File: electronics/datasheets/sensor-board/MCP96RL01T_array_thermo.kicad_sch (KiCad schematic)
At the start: 75 parts, among them J23 Therm_1, J24 Therm_4, J25 Therm_7, J26 Therm_2, J27 Therm_5, J28 Therm_3, J29 Therm_6, U10 MCP96RL01T, U4 MCP96RL01T, U5 MCP96RL01T, U6 MCP96RL01T, U7 MCP96RL01T, U8 MCP96RL01T, U9 MCP96RL01T

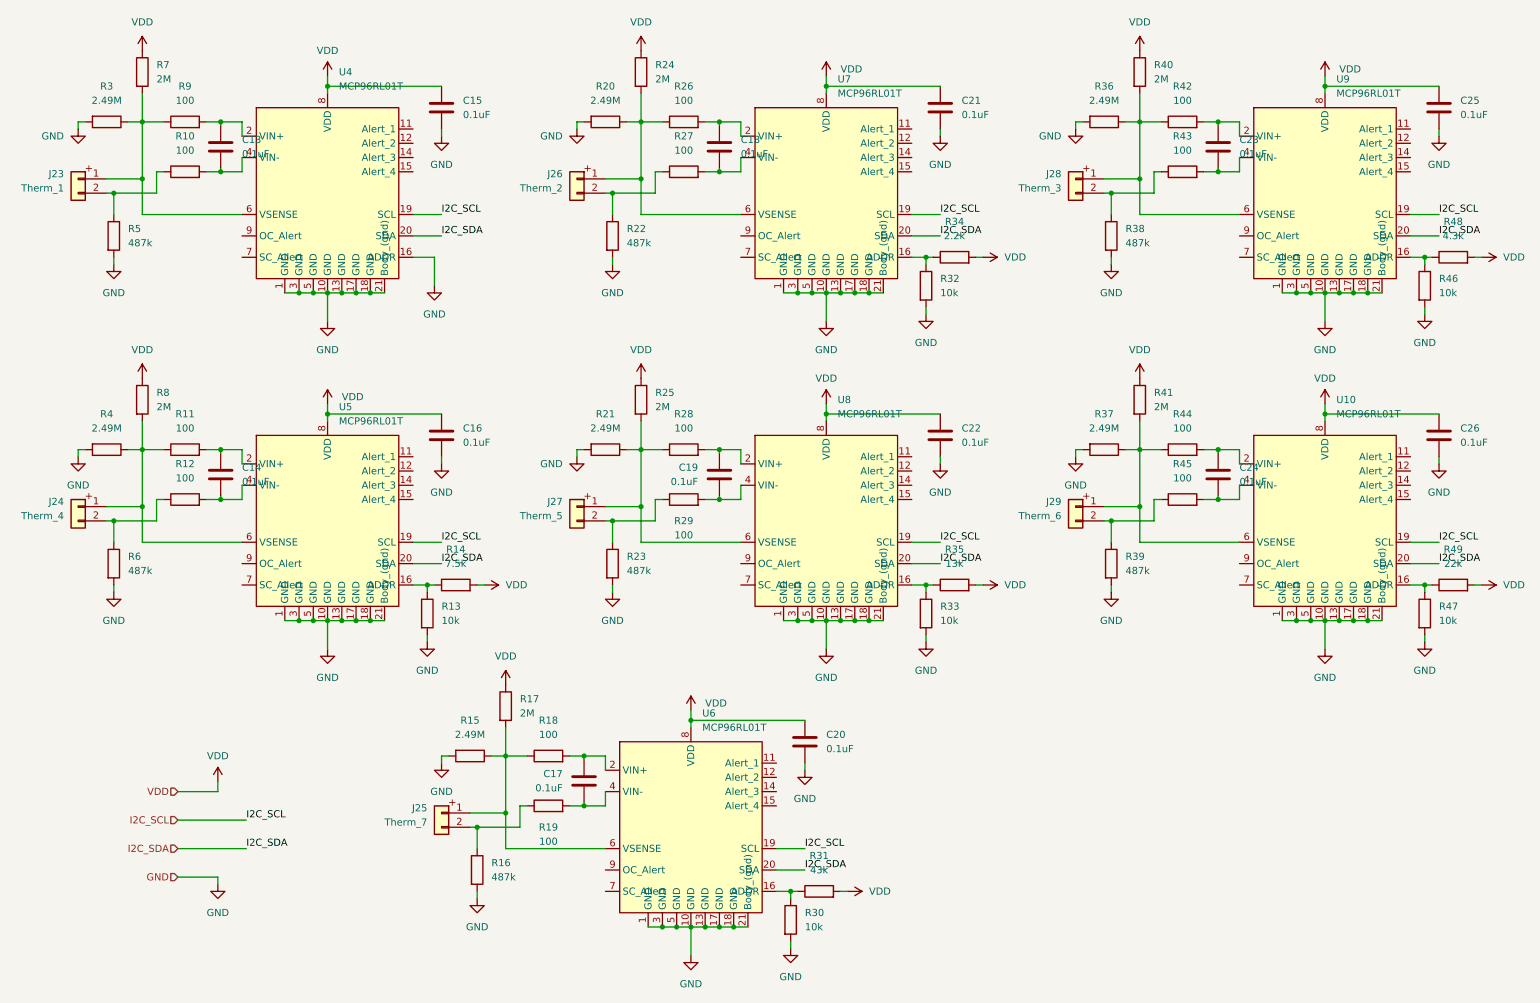
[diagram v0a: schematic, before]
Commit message: Work on sensor-board
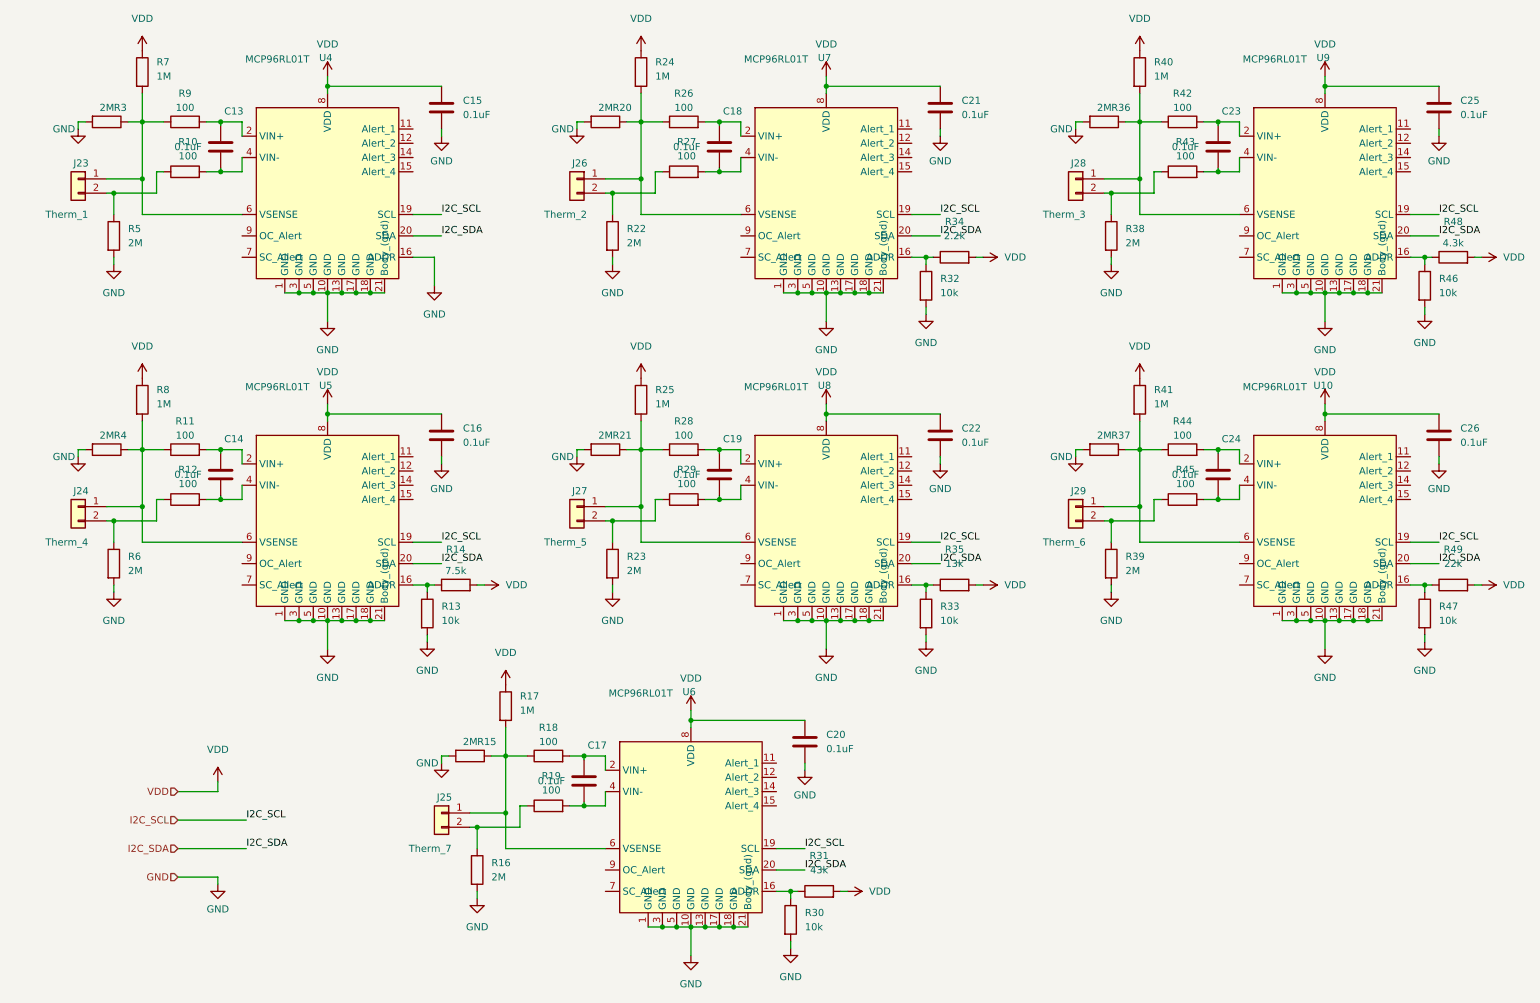
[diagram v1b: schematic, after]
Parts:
- J23, J24, J25, J26, J27, J28, J29: symbol K_type_thermo_conn_F:K_type_thermo_conn_F -> Connector_Generic:Conn_01x02
- R15, R20, R21, R3, R36, R37, R4: value 2.49M -> 2M
- R16, R22, R23, R38, R39, R5, R6: value 487k -> 2M
- R17, R24, R25, R40, R41, R7, R8: value 2M -> 1M
